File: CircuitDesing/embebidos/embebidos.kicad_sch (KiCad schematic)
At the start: 0 parts

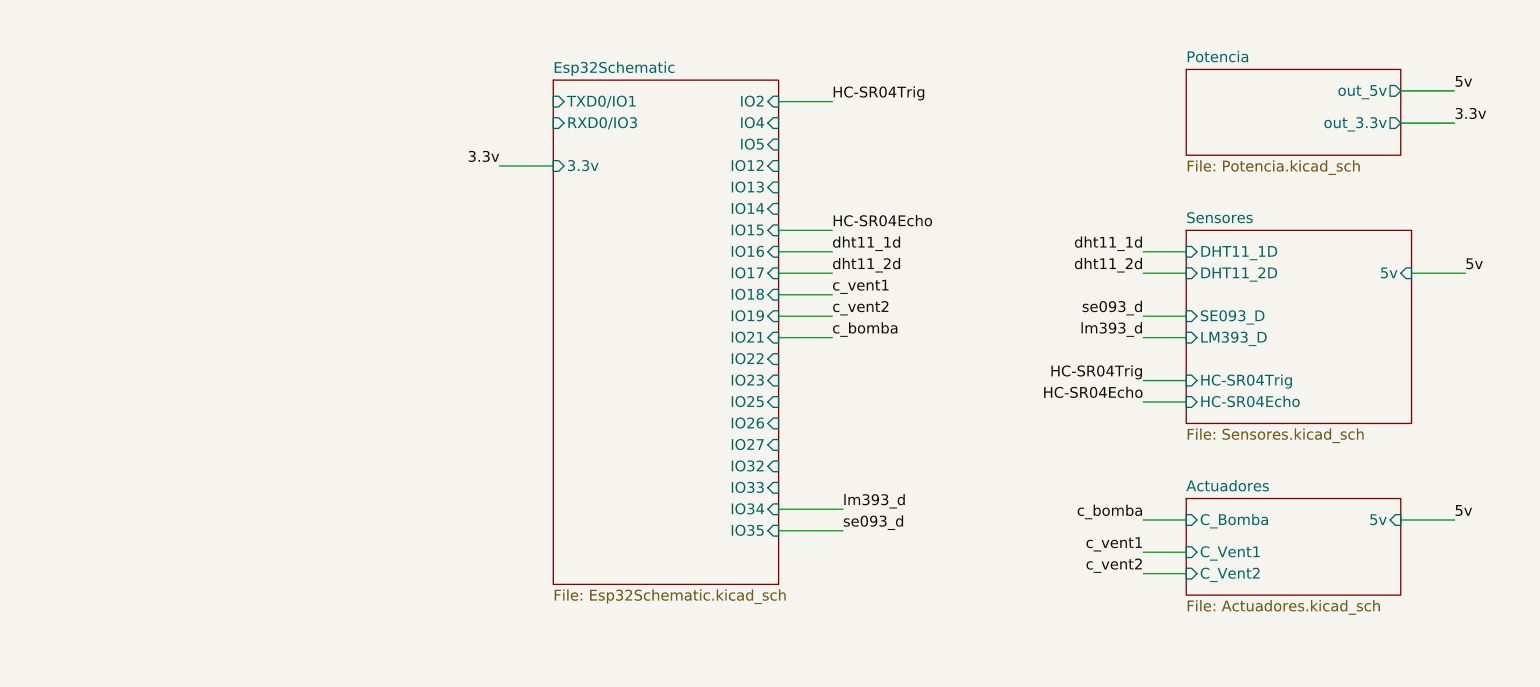
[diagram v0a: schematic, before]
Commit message: Actualizacion huellas
Huellas+Programador
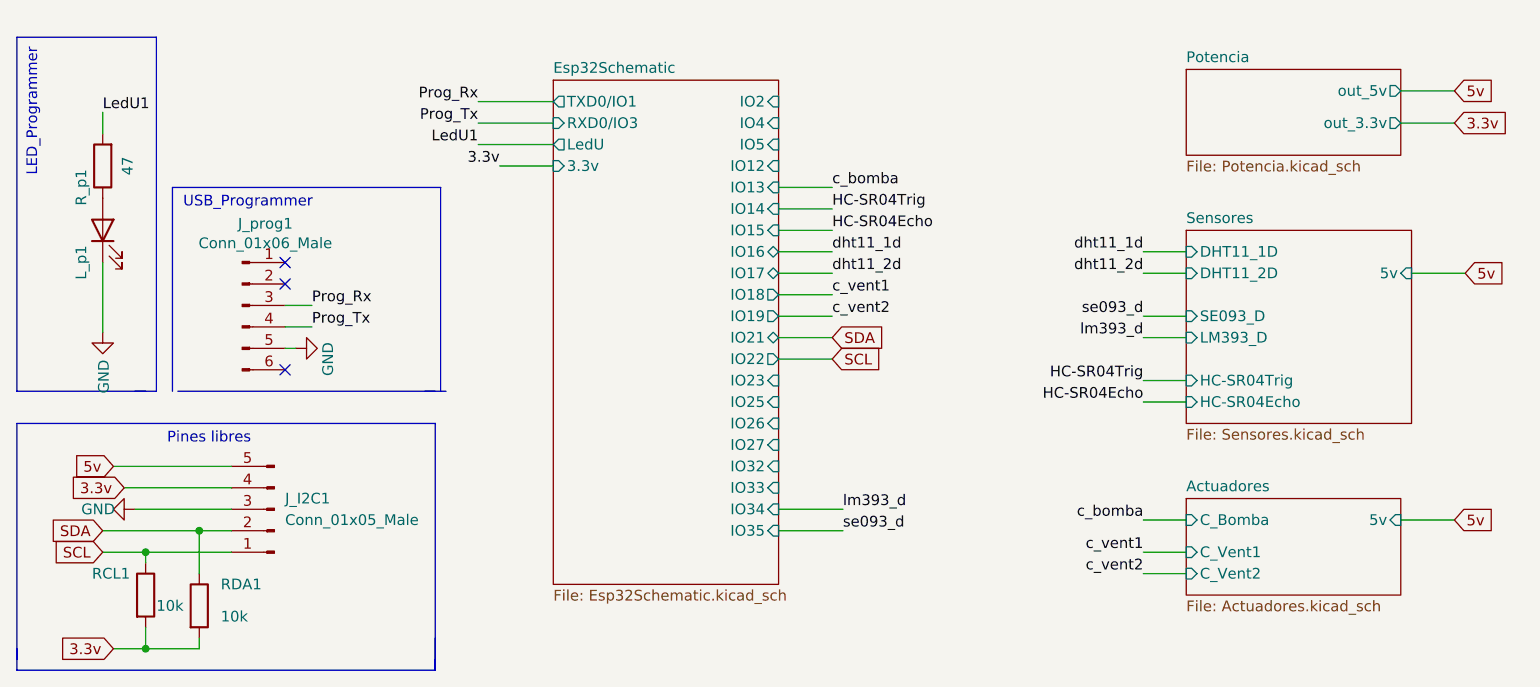
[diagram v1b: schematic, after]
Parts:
- added J_I2C1: Conn_01x05_Male, Connector_PinSocket_2.54mm:PinSocket_1x05_P2.54mm_Horizontal, symbol Connector:Conn_01x05_Male
- added J_prog1: Conn_01x06_Male, Connector_PinHeader_2.54mm:PinHeader_1x06_P2.54mm_Horizontal, symbol Connector:Conn_01x06_Male
- added L_p1: LED, LED_SMD:LED_0805_2012Metric_Pad1.15x1.40mm_HandSolder, symbol Device:LED
- added RCL1, RDA1: 10k, Resistor_SMD:R_0805_2012Metric_Pad1.20x1.40mm_HandSolder, symbol Device:R
- added R_p1: 47, Resistor_SMD:R_0805_2012Metric_Pad1.20x1.40mm_HandSolder, symbol Device:R
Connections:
- net 3.3v: now also J_I2C1.4 (Pin_4), RCL1.2, RDA1.2
- net 5v: now also J_I2C1.5 (Pin_5)
- new net: L_p1.2 (A), R_p1.1
- new net GND: J_I2C1.3 (Pin_3), J_prog1.5 (Pin_5), L_p1.1 (K)
- new net LedU1: R_p1.2
- new net Prog_Rx: J_prog1.3 (Pin_3)
- new net Prog_Tx: J_prog1.4 (Pin_4)
- new net SCL: J_I2C1.1 (Pin_1), RCL1.1
- new net SDA: J_I2C1.2 (Pin_2), RDA1.1
- no-connect marks 0 -> 3
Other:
- sheet Esp32Schematic ports: added LedU; removed none
- note added: "LED_Programmer"
- note added: "Pines libres"
- note added: "USB_Programmer"
